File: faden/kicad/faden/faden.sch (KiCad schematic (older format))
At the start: 33 parts, among them J1Power1 Conn_01x02_Male, J2Signal1 Conn_01x04_Male, SW1 SW_DPDT_x2, U1 TL082

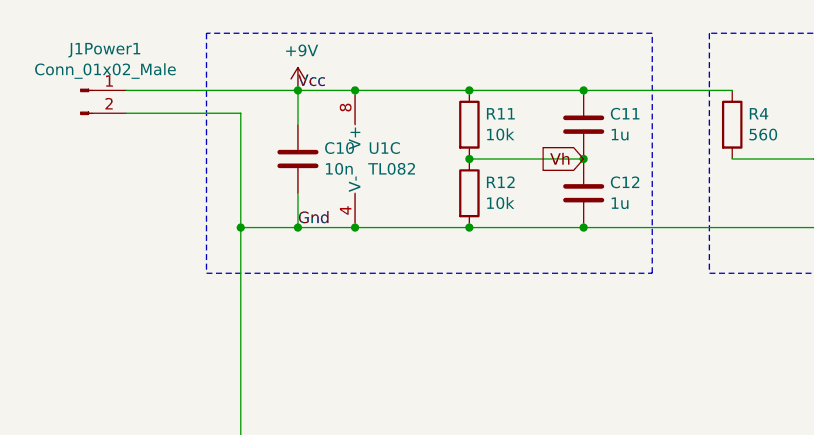
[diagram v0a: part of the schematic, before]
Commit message: final layout for strip layout
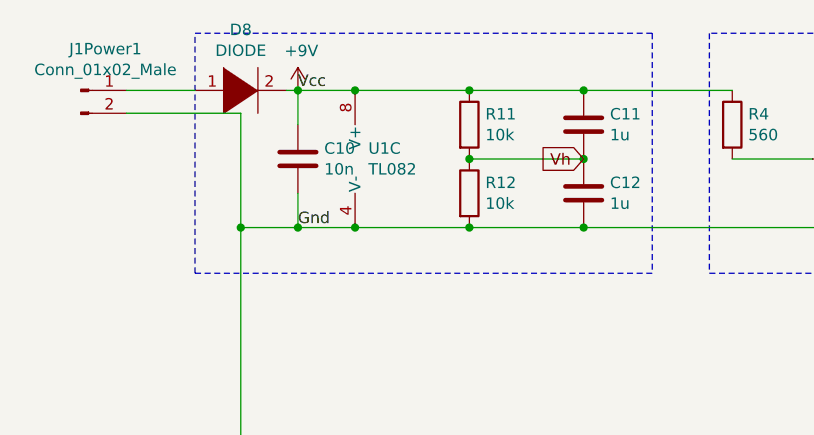
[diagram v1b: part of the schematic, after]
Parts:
- added D8: DIODE, Diode_THT:D_DO-15_P10.16mm_Horizontal, symbol pspice:DIODE
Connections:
- net +9V: now also D8.2 (A); no longer J1Power1.1 (Pin_1)
- new net: D8.1 (K), J1Power1.1 (Pin_1)
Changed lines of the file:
@@
 	1    0    0    -1
 $EndComp
-Wire Wire Line
-	1000 1500 1750 1500
 $Comp
 L Device:C C10
@@
 	7650 5500 5350 5500
 Connection ~ 5350 5500
-Wire Notes Line
-	1350 1250 1350 2300
-Wire Notes Line
-	1350 2300 3300 2300
-Wire Notes Line
-	3300 2300 3300 1250
-Wire Notes Line
-	3300 1250 1350 1250
 $Comp
 L Device:LED_Dual_CAC D3
@@
 	7250 4500 6450 4500
 Connection ~ 6450 4500
+$Comp
+L pspice:DIODE D8
+U 1 1 5F72D601
+P 1500 1500
+F 0 "D8" H 1500 1765 50  0000 C CNN
+F 1 "DIODE" H 1500 1674 50  0000 C CNN
+F 2 "Diode_THT:D_DO-15_P10.16mm_Horizontal" H 1500 1500 50  0001 C CNN
+F 3 "~" H 1500 1500 50  0001 C CNN
+	1    1500 1500
+	1    0    0    -1
+$EndComp
+Wire Wire Line
+	1000 1500 1300 1500
+Wire Wire Line
+	1700 1500 1750 1500
+Wire Notes Line
+	3300 2300 1300 2300
+Wire Notes Line
+	1300 2300 1300 1250
+Wire Notes Line
+	1300 1250 3300 1250
+Wire Notes Line
+	3300 1250 3300 2300
 $EndSCHEMATC
